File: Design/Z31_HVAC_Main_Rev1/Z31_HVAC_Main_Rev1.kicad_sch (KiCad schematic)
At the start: 24 parts, among them J1 Conn_01x05, J2 Conn_02x18_Odd_Even, J3 Conn_01x10_Male, J4 Conn_01x09_Male, U1 MEGA2560PRO, U2 MCP2515, U3 TJR1443, U4 ULN2003, U5 ULN2003, U6 ULN2003, U7 ULN2003, U8 NCV4276B, U9 ULN2003

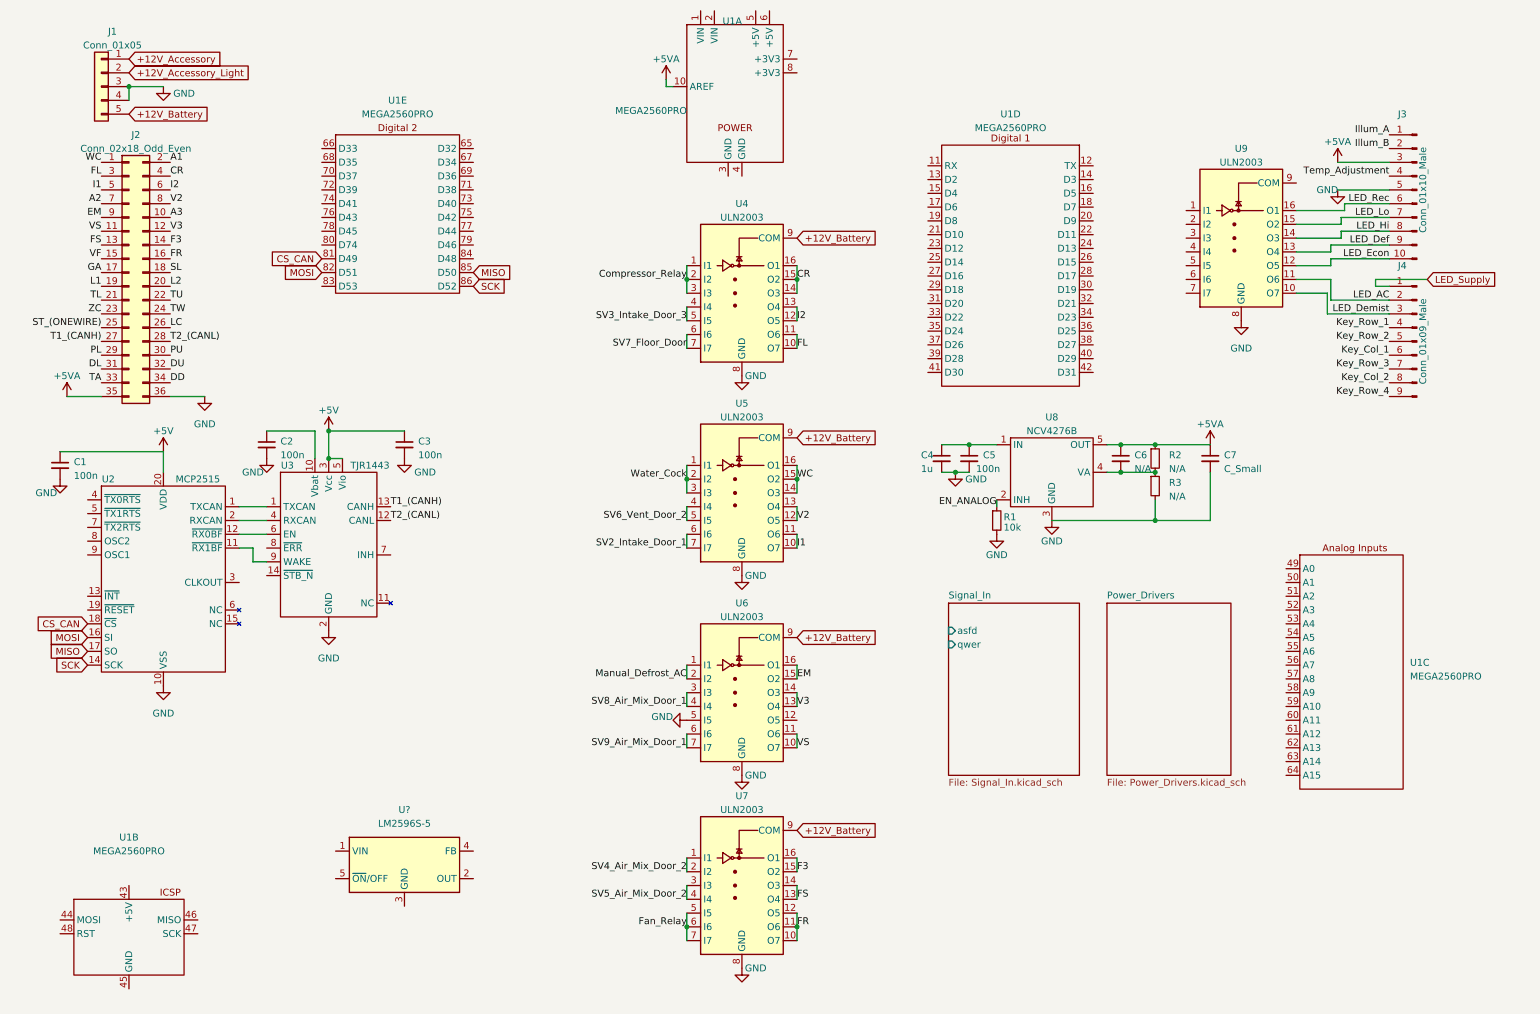
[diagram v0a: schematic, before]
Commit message: large changes
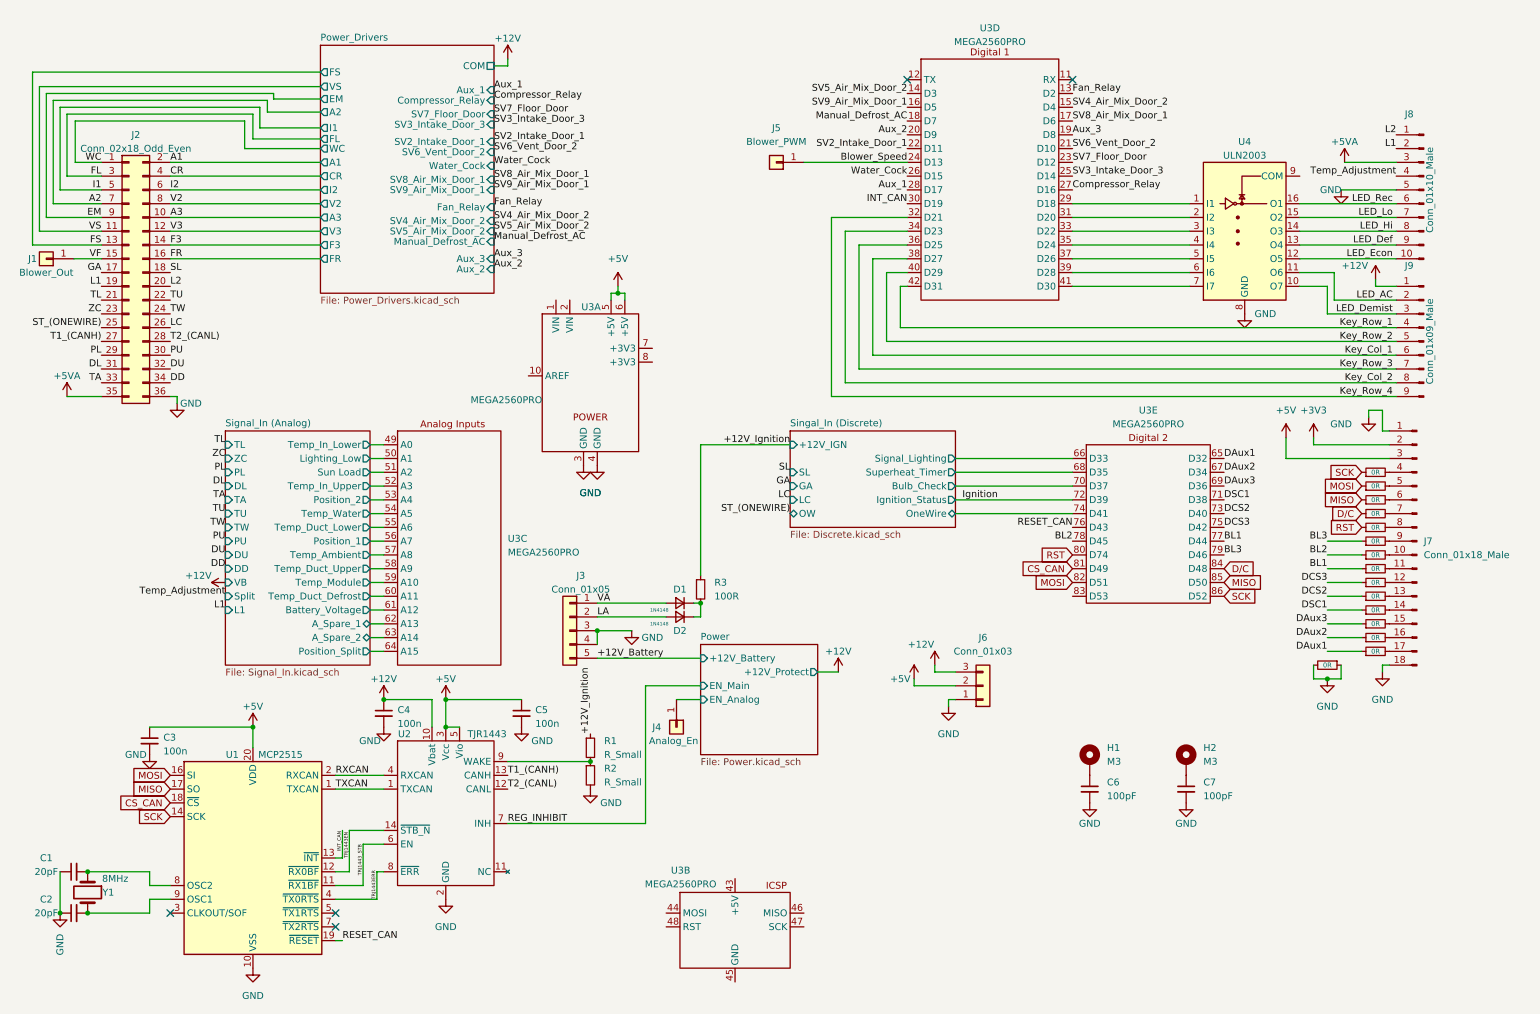
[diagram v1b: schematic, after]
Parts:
- removed C4: 1u, Capacitor_SMD:C_1210_3225Metric_Pad1.33x2.70mm_HandSolder, symbol Device:C_Small
- removed C5: 100n, Capacitor_SMD:C_0805_2012Metric_Pad1.18x1.45mm_HandSolder, symbol Device:C_Small
- removed U4, U5, U6, U7: ULN2003, Package_SO:SO-16_3.9x9.9mm_P1.27mm, symbol Transistor_Array:ULN2003
- removed U8: NCV4276B, Package_TO_SOT_SMD:TO-263-5_TabPin3, symbol Personal:NCV4276B
- removed U?: LM2596S-5, Package_TO_SOT_SMD:TO-263-5_TabPin3, symbol Regulator_Switching:LM2596S-5
- added C1, C2: 20pF, Capacitor_SMD:C_0805_2012Metric_Pad1.18x1.45mm_HandSolder, symbol Device:C_Small
- added D1, D2: 1N4148, Diode_SMD:D_SOD-323_HandSoldering, symbol Device:D_Small
- added H1, H2: M3, MountingHole:MountingHole_3.5mm_Pad, symbol Mechanical:MountingHole_Pad
- added J1: Blower_Out, Connector_PinHeader_2.54mm:PinHeader_1x01_P2.54mm_Vertical, symbol Connector_Generic:Conn_01x01
- added J4: Analog_En, Connector_PinHeader_2.54mm:PinHeader_1x01_P2.54mm_Vertical, symbol Connector_Generic:Conn_01x01
- added J5: Blower_PWM, Connector_PinHeader_2.54mm:PinHeader_1x01_P2.54mm_Vertical, symbol Connector_Generic:Conn_01x01
- added J6: Conn_01x03, Personal:Proto-Area, symbol Connector_Generic:Conn_01x03
- added J7: Conn_01x18_Male, Connector_PinHeader_2.54mm:PinHeader_1x18_P2.54mm_Vertical, symbol Connector:Conn_01x18_Male
- added R10, R11, R12, R13, R14, R15, R16, R17, R18, R4, R5, R6, R7, R8, R9: 0R, Resistor_THT:R_Axial_DIN0204_L3.6mm_D1.6mm_P2.54mm_Vertical, symbol Device:R_Small
- added Y1: 8MHz, Crystal:Crystal_SMD_HC49-SD, symbol Device:Crystal
- C6: value N/A -> 100pF
- C7: value C_Small -> 100pF; footprint Capacitor_SMD:C_1210_3225Metric_Pad1.33x2.70mm_HandSolder -> Capacitor_SMD:C_0805_2012Metric_Pad1.18x1.45mm_HandSolder
- J2: footprint Personal:z31_hvac_connector_2 -> Personal:TE-172023
- J3: renamed from J1; footprint (none) -> Personal:Z31_HVAC_Connector_1
- R1: value 10k -> R_Small
- R2: value N/A -> R_Small
- R3: value N/A -> 100R; footprint Resistor_SMD:R_0805_2012Metric_Pad1.20x1.40mm_HandSolder -> Resistor_THT:R_Axial_DIN0207_L6.3mm_D2.5mm_P7.62mm_Horizontal
- U1: renamed from U2; symbol Personal:MCP2510 -> Interface_CAN_LIN:MCP2515-xST
- renumbered C1 to C3, C2 to C4, C3 to C5, J3 to J8, J4 to J9, U3 to U2, U1 to U3, U9 to U4
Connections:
- net Illum_A is gone; now on net L2: J8.1 (Pin_1)
- net Illum_B is gone; now on net L1: J8.2 (Pin_2)
- net LED_Supply is gone; now on net +12V: J9.1 (Pin_1)
- net +5V: now also U3.5 (+5V), U3.6 (+5V), J6.2 (Pin_2), J7.3 (Pin_3)
- net +5VA: no longer C6.1, C7.1, R2.1, U3.10 (AREF)
- net Compressor_Relay: now also U3.27 (D16)
- net Fan_Relay: now also U3.13 (D2)
- net GND: now also C6.2, R2.2, U3.3 (GND), U3.4 (GND), C1.1, C2.1, J6.1 (Pin_1), J7.1 (Pin_1), J7.18 (Pin_18), R4.1, R4.2; no longer R1.2, R3.2
- net Key_Col_1: now also U3.38 (D27)
- net Key_Col_2: now also U3.34 (D23)
- net Key_Row_1: now also U3.42 (D31)
- net Key_Row_2: now also U3.40 (D29)
- net Key_Row_3: now also U3.36 (D25)
- net Key_Row_4: now also U3.32 (D21)
- net MISO: now also R7.1
- net MOSI: now also R6.1
- net Manual_Defrost_AC: now also U3.18 (D7)
- net SCK: now also R5.1
- net SV2_Intake_Door_1: now also U3.22 (D11)
- net SV3_Intake_Door_3: now also U3.25 (D14)
- net SV4_Air_Mix_Door_2: now also U3.15 (D4)
- net SV5_Air_Mix_Door_2: now also U3.14 (D3)
- net SV6_Vent_Door_2: now also U3.21 (D10)
- net SV7_Floor_Door: now also U3.23 (D12)
- net SV8_Air_Mix_Door_1: now also U3.17 (D6)
- net SV9_Air_Mix_Door_1: now also U3.16 (D5)
- net VF: now also J1.1 (Pin_1)
- net Water_Cock: now also U3.26 (D15)
- net TXCAN: now reaches U1.1 (TXCAN), U2.1 (TXCAN)
- net at U2.9 (WAKE): now also R1.2, R2.1; no longer U1.11 (~{RX1BF})
- net TRJ1443EN: now reaches U1.12 (~{RX0BF})
- net TRJ1443EN: now also U2.14 (~{STB_N}); no longer U2.6 (EN)
- net INT_CAN: now reaches U1.13 (~{INT})
- net INT_CAN: now also U3.30 (D19)
- net RESET_CAN: now reaches U1.19 (~{RESET})
- net RESET_CAN: now also U3.76 (D43)
- net RXCAN: now reaches U1.2 (RXCAN), U2.4 (RXCAN)
- net TRJ1443ERR: now reaches U1.4 (~{TX0RTS})
- net TRJ1443ERR: now also U2.8 (~{ERR})
- net at U1.8 (OSC2): now also C1.2, Y1.1
- net at U1.9 (OSC1): now also C2.2, Y1.2
- net +12V: now reaches C4.1, U2.10 (Vbat)
- net +12V: now also J6.3 (Pin_3)
- net REG_INHIBIT: now reaches U2.7 (INH)
- net Signal_In (Analog)/Temp_In_Lower: now reaches U3.49 (A0)
- net Signal_In (Analog)/Lighting_Low: now reaches U3.50 (A1)
- net Signal_In (Analog)/Sun Load: now reaches U3.51 (A2)
- net Signal_In (Analog)/Temp_In_Upper: now reaches U3.52 (A3)
- net Signal_In (Analog)/Position_2: now reaches U3.53 (A4)
- net Signal_In (Analog)/Temp_Water: now reaches U3.54 (A5)
- net Signal_In (Analog)/Temp_Duct_Lower: now reaches U3.55 (A6)
- net Signal_In (Analog)/Position_1: now reaches U3.56 (A7)
- net Signal_In (Analog)/Temp_Ambient: now reaches U3.57 (A8)
- net Signal_In (Analog)/Temp_Duct_Upper: now reaches U3.58 (A9)
- net Signal_In (Analog)/Temp_Module: now reaches U3.59 (A10)
- net Signal_In (Analog)/Temp_Duct_Defrost: now reaches U3.60 (A11)
- net Signal_In (Analog)/Battery_Voltage: now reaches U3.61 (A12)
- net Signal_In (Analog)/A_Spare_1: now reaches U3.62 (A13)
- net Signal_In (Analog)/A_Spare_2: now reaches U3.63 (A14)
- net Signal_In (Analog)/Position_Split: now reaches U3.64 (A15)
- net Aux_3: now reaches U3.19 (D8)
- net Aux_2: now reaches U3.20 (D9)
- net Blower_Speed: now reaches U3.24 (D13)
- net Blower_Speed: now also J5.1 (Pin_1)
- net Aux_1: now reaches U3.28 (D17)
- net at U3.29 (D18): now also U4.1 (I1)
- net at U3.31 (D20): now also U4.2 (I2)
- net at U3.33 (D22): now also U4.3 (I3)
- net at U3.35 (D24): now also U4.4 (I4)
- net at U3.37 (D26): now also U4.5 (I5)
- net at U3.39 (D28): now also U4.6 (I6)
- net at U3.41 (D30): now also U4.7 (I7)
- net DAux1: now reaches U3.65 (D32)
- net DAux1: now also R18.1
- net Singal_In (Discrete)/Signal_Lighting: now reaches U3.66 (D33)
- net DAux2: now reaches U3.67 (D34)
- net DAux2: now also R17.1
- net Singal_In (Discrete)/Superheat_Timer: now reaches U3.68 (D35)
- net DAux3: now reaches U3.69 (D36)
- net DAux3: now also R16.1
- net Singal_In (Discrete)/Bulb_Check: now reaches U3.70 (D37)
- net DSC1: now reaches U3.71 (D38)
- net DSC1: now also R15.1
- net Ignition: now reaches U3.72 (D39)
- net DCS2: now reaches U3.73 (D40)
- net DCS2: now also R14.1
- net Singal_In (Discrete)/OneWire: now reaches U3.74 (D41)
- net DCS3: now reaches U3.75 (D42)
- net DCS3: now also R13.1
- net BL1: now reaches U3.77 (D44)
- net BL1: now also R12.1
- net BL2: now reaches U3.78 (D45)
- net BL2: now also R11.1
- net BL3: now reaches U3.79 (D46)
- net BL3: now also R10.1
- net RST: now reaches U3.80 (D74)
- net RST: now also R9.1
- net D/C: now reaches U3.84 (D48)
- net D/C: now also R8.1
- net +12V_Accessory renamed VA
- net VA: now also D1.2 (A)
- net +12V_Accessory_Light renamed LA
- net LA: now also D2.2 (A)
- net EN_ANALOG renamed +12V_Ignition
- net +12V_Ignition: now also R3.1
- new net: J7.11 (Pin_11), R12.2
- new net: J7.4 (Pin_4), R5.2
- new net: J7.17 (Pin_17), R18.2
- new net: J7.6 (Pin_6), R7.2
- new net: D1.1 (K), D2.1 (K), R3.2
- new net: J7.5 (Pin_5), R6.2
- new net: C7.1, H2.1
- new net: J7.9 (Pin_9), R10.2
- new net: J7.16 (Pin_16), R17.2
- new net: C6.1, H1.1
- new net: J7.10 (Pin_10), R11.2
- new net: J7.12 (Pin_12), R13.2
- new net: J7.13 (Pin_13), R14.2
- new net: J7.14 (Pin_14), R15.2
- new net: J7.15 (Pin_15), R16.2
- new net: J7.7 (Pin_7), R8.2
- new net: J7.8 (Pin_8), R9.2
- new net +3V3: J7.2 (Pin_2)
- new net Power/EN_Analog: J4.1 (Pin_1)
- new net TRJ1443_STB: U1.11 (~{RX1BF}), U2.6 (EN)
- no-connect marks 0 -> 5
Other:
- sheet Signal_In renamed Signal_In (Analog)
- added sheet Power (Power.kicad_sch)
- added sheet Singal_In (Discrete) (Discrete.kicad_sch)
- sheet Power_Drivers ports: added A1, A2, A3, Aux_1, Aux_2, Aux_3, COM, CR, Compressor_Relay, EM, F3, FL, FR, FS, Fan_Relay, I1, I2, Manual_Defrost_AC, SV2_Intake_Door_1, SV3_Intake_Door_3, SV4_Air_Mix_Door_2, SV5_Air_Mix_Door_2, SV6_Vent_Door_2, SV7_Floor_Door, SV8_Air_Mix_Door_1, SV9_Air_Mix_Door_1, V2, V3, VS, WC, Water_Cock; removed none
- sheet Signal_In (Analog) ports: added A_Spare_1, A_Spare_2, Battery_Voltage, DD, DL, DU, L1, Lighting_Low, PL, PU, Position_1, Position_2, Position_Split, Split, Sun Load, TA, TL, TU, TW, Temp_Ambient, Temp_Duct_Defrost, Temp_Duct_Lower, Temp_Duct_Upper, Temp_In_Lower, Temp_In_Upper, Temp_Module, Temp_Water, VB, ZC; removed asfd, qwer
- moved on the sheet: C3, C4, C5, J3, J8, J9, U2, U3A, U3B, U3C, U3D, U3E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
